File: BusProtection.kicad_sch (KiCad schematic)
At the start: 102 parts, among them Q1 MMBT2907, Q10 BSS138DWQ-7, Q11 BSS138DWQ-7, Q12 MBT2222ADW1T1, Q13 MBT2222ADW1T1, Q14 BSS138DWQ-7, Q15 BSS138DWQ-7, Q16 MBT2222ADW1T1, Q17 MBT2222ADW1T1, Q18 MMBT2907, Q2 BSS138DWQ-7, Q20 BSS138DWQ-7, Q21 MBT2222ADW1T1, Q22 BSS138DWQ-7, Q23 MBT2222ADW1T1, Q3 BSS138DWQ-7, Q4 MBT2222ADW1T1, Q5 MBT2222ADW1T1, Q6 BSS138DWQ-7, Q7 BSS138DWQ-7, Q8 MBT2222ADW1T1, Q9 MBT2222ADW1T1

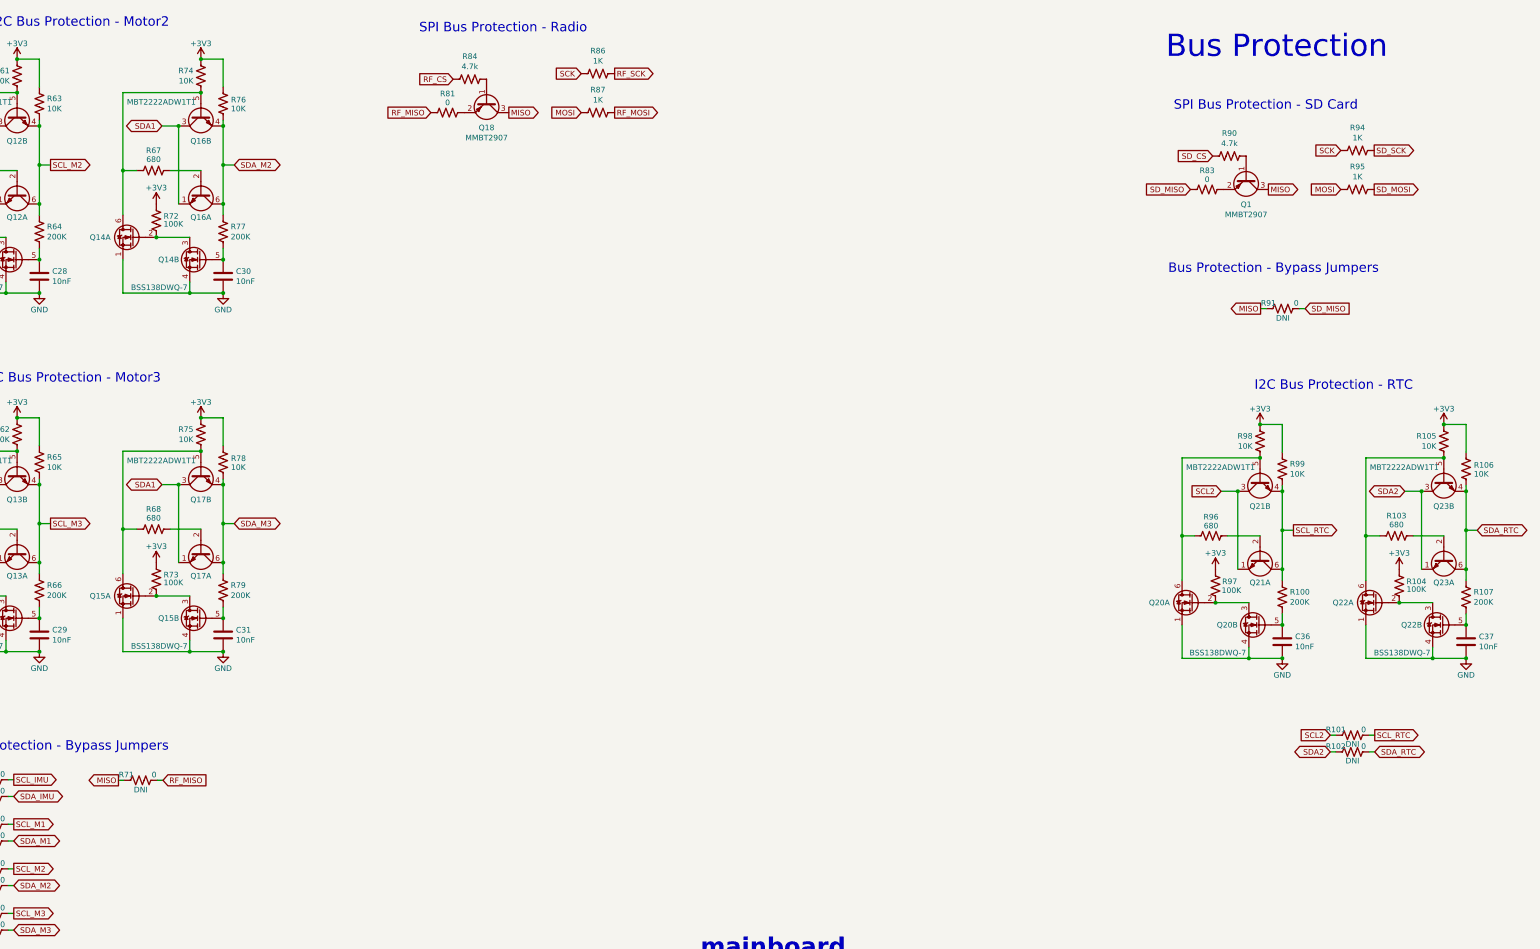
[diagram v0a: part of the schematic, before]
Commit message: Some fixes
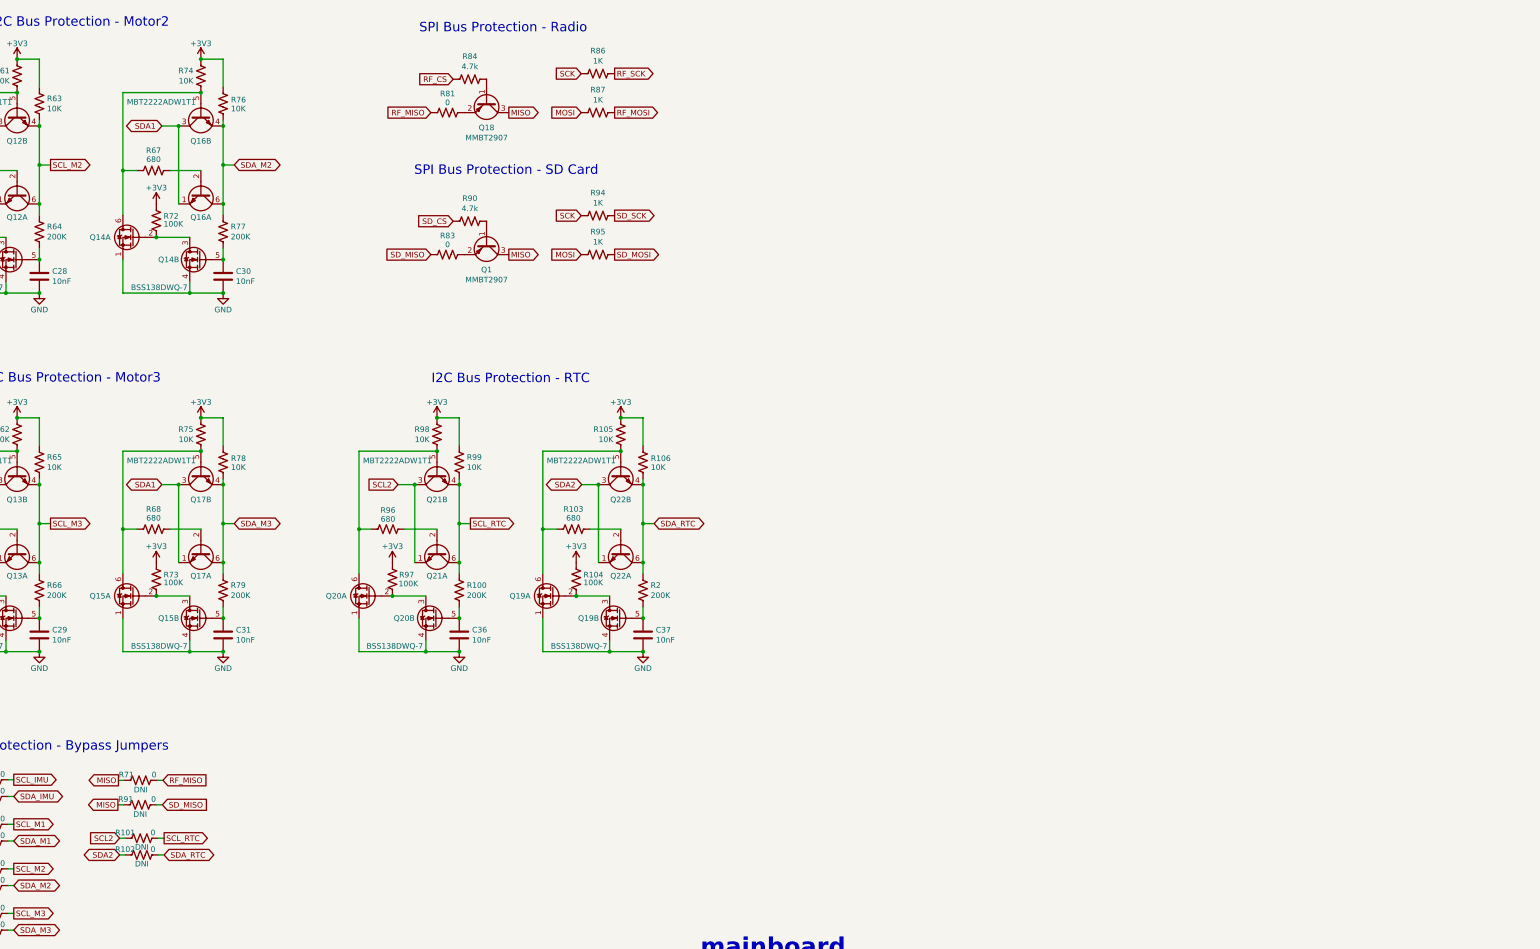
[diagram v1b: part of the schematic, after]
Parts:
- renumbered Q22 to Q19, Q23 to Q22, R107 to R2
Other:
- note removed: "Bus Protection"
- moved on the sheet: C36, C37, Q1, Q19A, Q19B, Q20A, Q20B, Q21A, Q21B, Q22A, Q22B, R100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

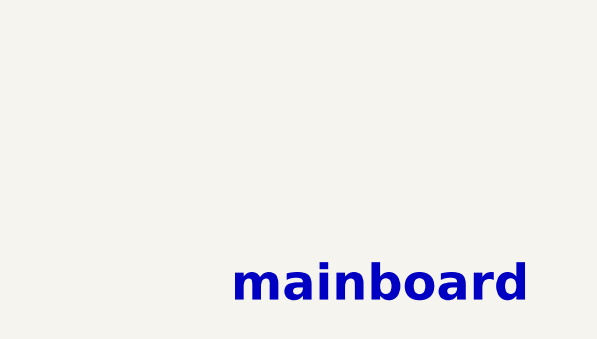
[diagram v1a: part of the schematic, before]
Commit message: Finished B2/01 Updates
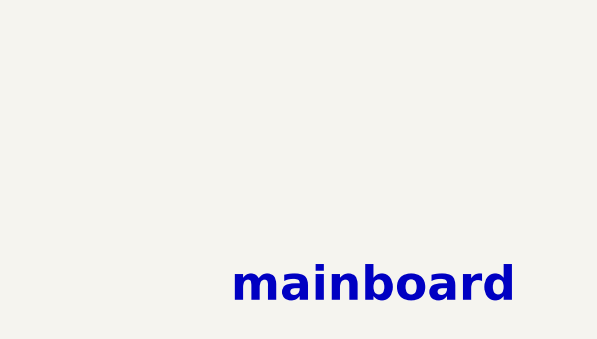
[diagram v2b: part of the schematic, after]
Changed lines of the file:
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@@
   (title_block
     (title "PyCubed Mini")
-    (date "2022-09-06")
-    (rev "B1/04")
+    (date "2022-10-09")
+    (rev "B2/01")
     (company "RExLab Carnegie Mellon University")
     (comment 1 "Z. Manchester")
@@
   )
   (text "mainboard" (at 350.393 245.872 0)
-    (effects (font (size 3.9878 3.9878) (thickness 0.7976) bold) (justify left bottom))
+    (effects (font (size 3.81 3.81) (thickness 0.7976) bold) (justify left bottom))
   )
   (text "SPI Bus Protection - Radio" (at 286.258 35.052 0)
